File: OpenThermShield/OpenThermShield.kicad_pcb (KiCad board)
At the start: 2 copper layers, 55 x 118.5 mm, 27 parts, among them J1 Screw_Terminal_01x02, Q1 BC558, U1 WEMOS_D1_mini, U2 Optocoupler_DC_PhotoNPN_AKEC, U3 Optocoupler_DC_PhotoNPN_AKEC

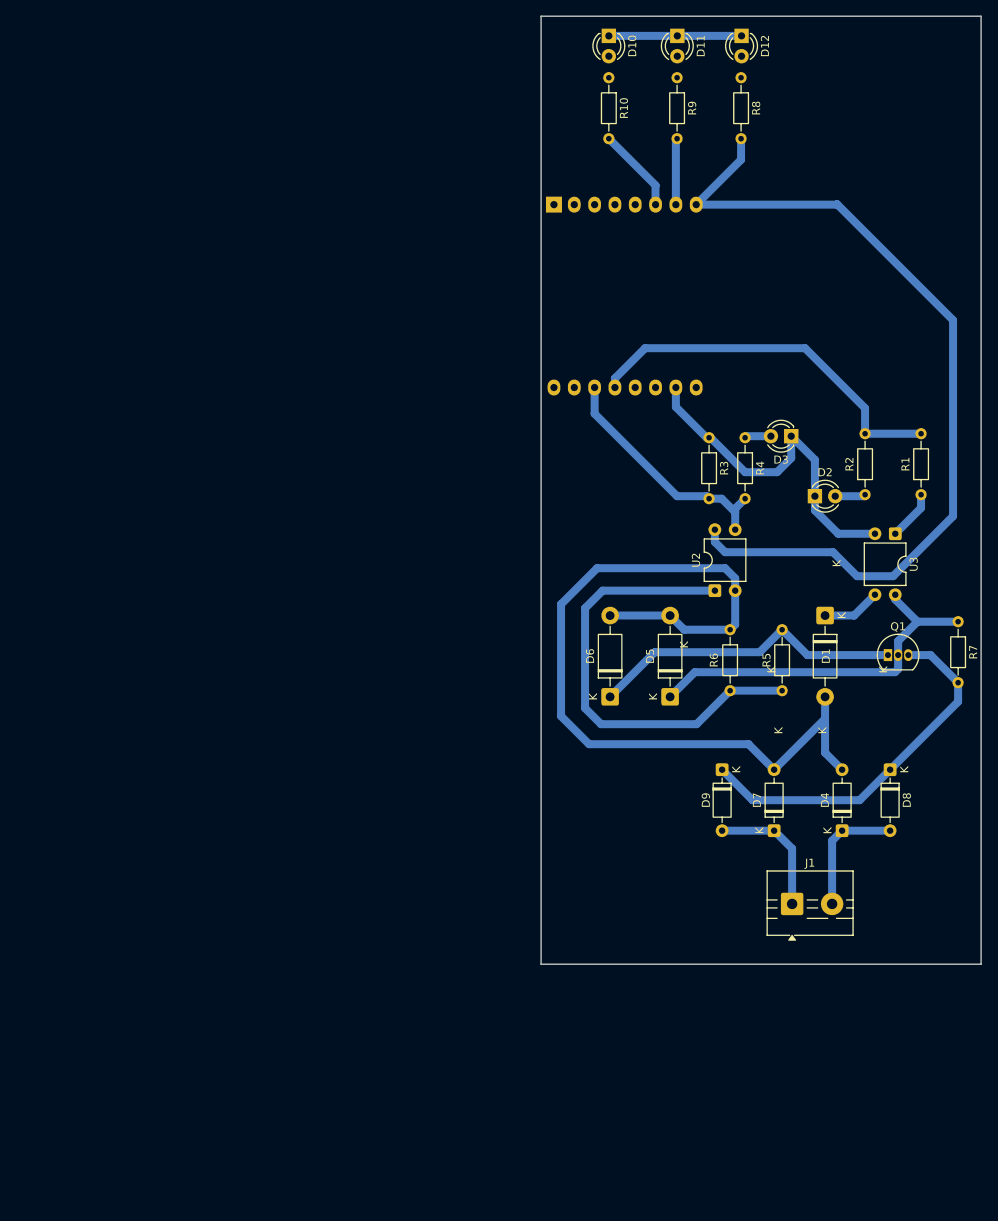
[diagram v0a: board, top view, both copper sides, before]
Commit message: docs
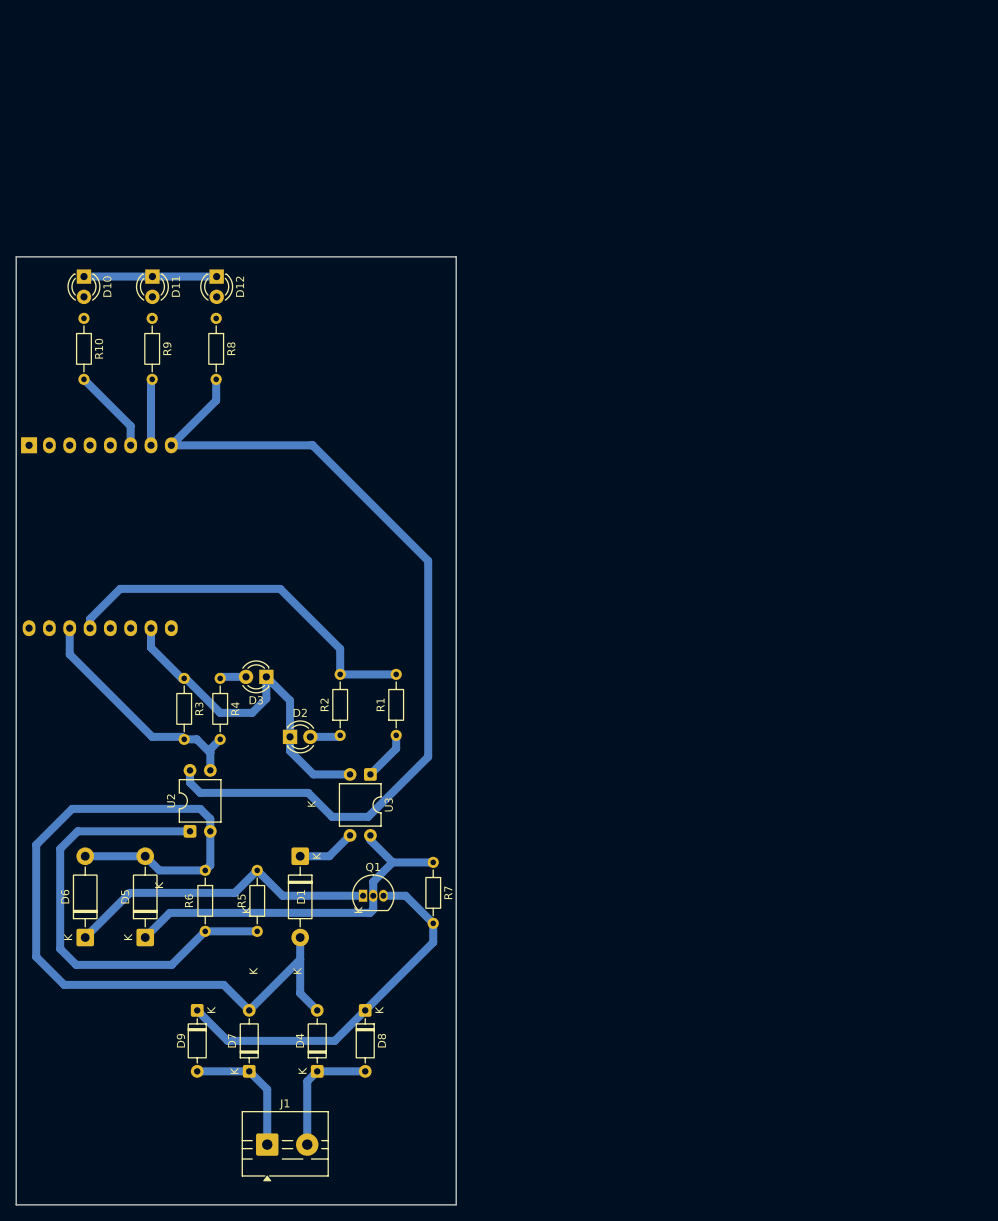
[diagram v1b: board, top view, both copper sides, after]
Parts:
- moved D2 72.2 mm to (55.1, 134.6)
- moved Q1 72.2 mm to (64.2, 154.4)
- moved D1 72.2 mm to (56.4, 149.5)
- moved D10 72.2 mm to (29.4, 77.0)
- moved D11 72.2 mm to (37.9, 77.0)
- moved D12 72.2 mm to (46.0, 77.0)
- moved D3 72.2 mm to (52.2, 127.1)
- moved D4 72.2 mm to (58.5, 176.4)
- moved D6 72.2 mm to (29.5, 159.7)
- moved D7 72.2 mm to (50.0, 176.4)
- moved D8 72.2 mm to (64.5, 168.8)
- moved D9 72.2 mm to (43.5, 168.8)
- moved J1 72.2 mm to (52.3, 185.6)
- moved R1 72.2 mm to (68.4, 134.4)
- moved R10 72.2 mm to (29.4, 82.3)
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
